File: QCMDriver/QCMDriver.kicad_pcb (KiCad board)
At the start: 2 copper layers, 43 x 34 mm, 28 parts, among them J1 Conn_Coaxial, J2 Conn_Coaxial, J3 Conn_Coaxial, Q1 BC817, U1 74LVC1GU04DRL, U2 74LVC1GU04DRL

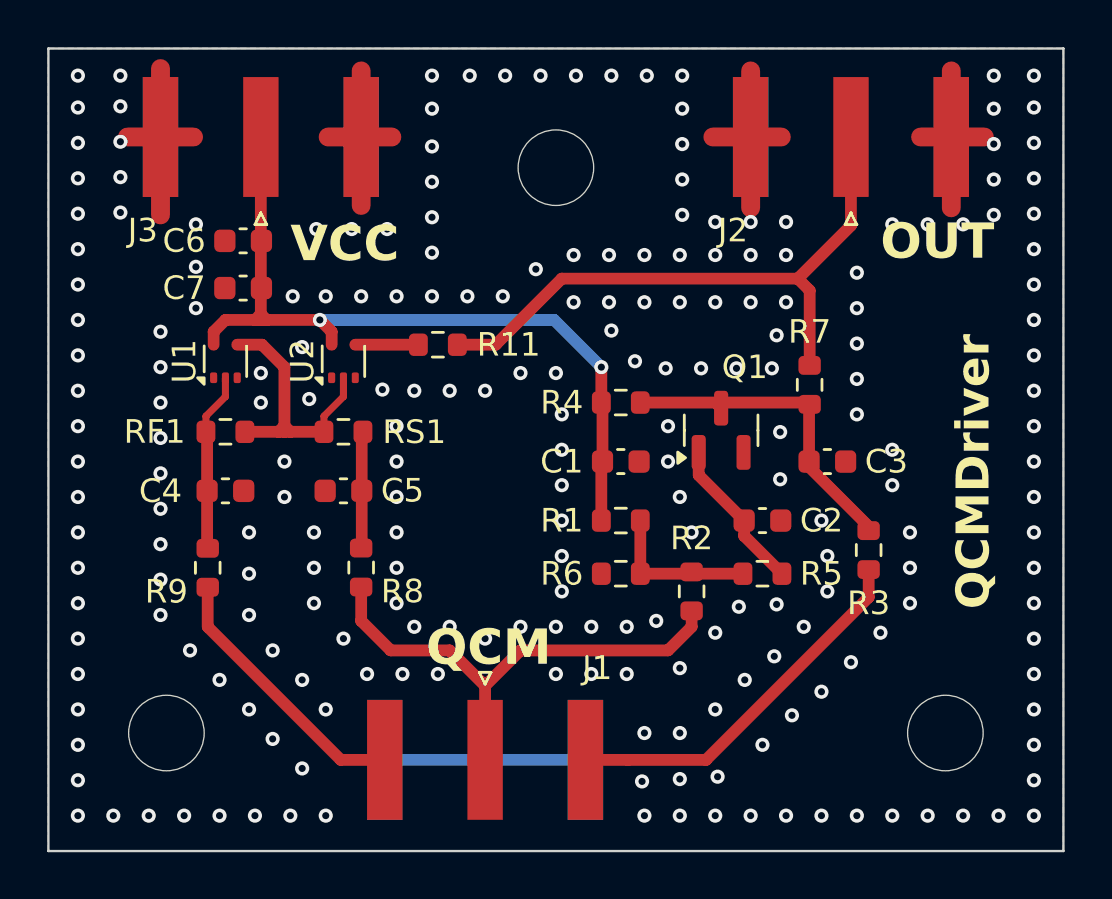
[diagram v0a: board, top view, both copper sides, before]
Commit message: misc improvements
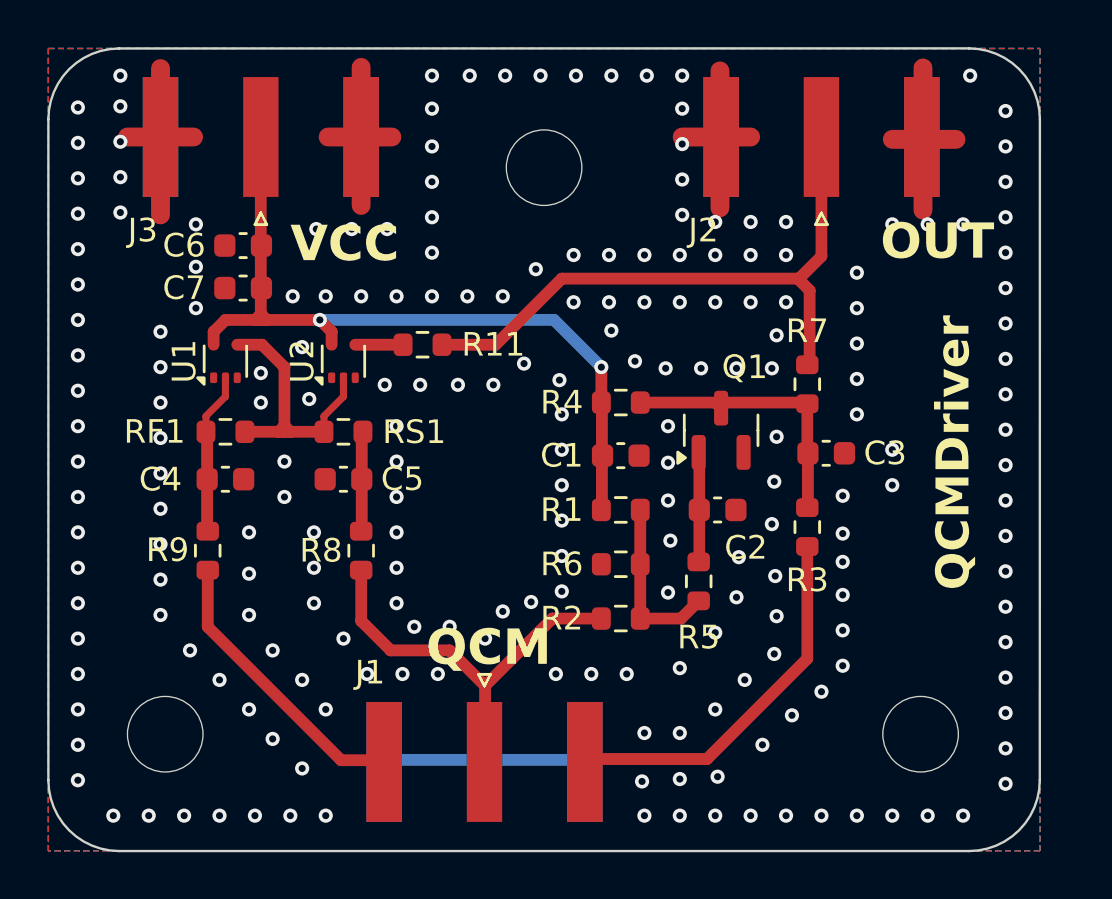
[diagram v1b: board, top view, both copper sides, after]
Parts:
- moved R2 3.21 mm to (128.5, 108.4), turned to 0 degrees
- moved R3 2.78 mm to (136.4, 104.5)
- moved R5 2.72 mm to (131.8, 106.8), turned to 90 degrees
- moved C2 1.95 mm to (132.6, 103.8)
- moved J2 1.25 mm to (137.0, 88.0)
- moved H1 1.05 mm to (141.2, 113.3)
- moved R9 0.72 mm to (111.0, 105.5)
- moved R8 0.71 mm to (117.5, 105.5)
- moved R11 0.65 mm to (120.1, 96.8)
- moved H2 0.50 mm to (125.2, 89.3)
- moved C4 0.49 mm to (111.8, 102.5)
- moved C5 0.49 mm to (116.8, 102.5)
- moved R1 0.45 mm to (128.5, 103.8)
- moved R6 0.40 mm to (128.5, 106.1)
- moved C3 0.35 mm to (137.2, 101.4)
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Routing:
- net /QCMA: track 21.4 -> 17.8 mm
- net Net-(Q1-C): track 14.1 -> 11.8 mm
- net Net-(Q1-B): track 6.60 -> 4.68 mm
- net /OUT_OSC: track 25.0 -> 26.6 mm
- net VCCOSC: track 33.0 -> 32.3 mm
- net Net-(R11-Pad1): track 2.76 -> 2.03 mm
- net Net-(C4-Pad1): track 7.60 -> 6.87 mm
- net Net-(R1-Pad2): track 6.66 -> 7.39 mm
- net Net-(C5-Pad1): track 4.96 -> 4.24 mm
- net /QCMB: track 36.0 -> 36.7 mm
- net GND: track 34.8 -> 35.0 mm, vias 229 -> 218
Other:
- board size 43 x 34 mm -> 42 x 34 mm
- board text added: "JLCJLCJLCJLC"
